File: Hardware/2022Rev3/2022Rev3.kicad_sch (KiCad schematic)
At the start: 101 parts, among them J1 Conn_01x04, J2 Conn_01x06, J3 RJ45_LED_Shielded, J4 Conn_01x09, J5 Conn_01x09, J6 Conn_01x03, Q1 Q_NMOS_DGS, Q2 Q_NMOS_DGS, SW1 SW_SPDT, U1 ACS758xCB-200B-PFF, U2 LT1910, U3 TRS12433, U4 TRS12450, U5 Teensy4.1_DEV-16771, U6 Opamp_Dual, U7 Opamp_Dual, U8 Opamp_Dual, U9 Opamp_Dual

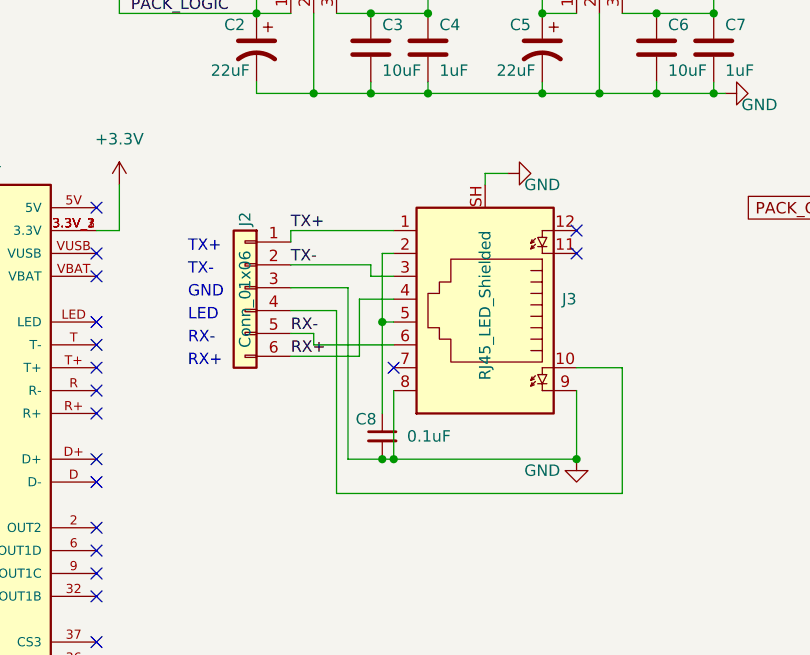
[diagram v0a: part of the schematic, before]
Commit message: layout changes
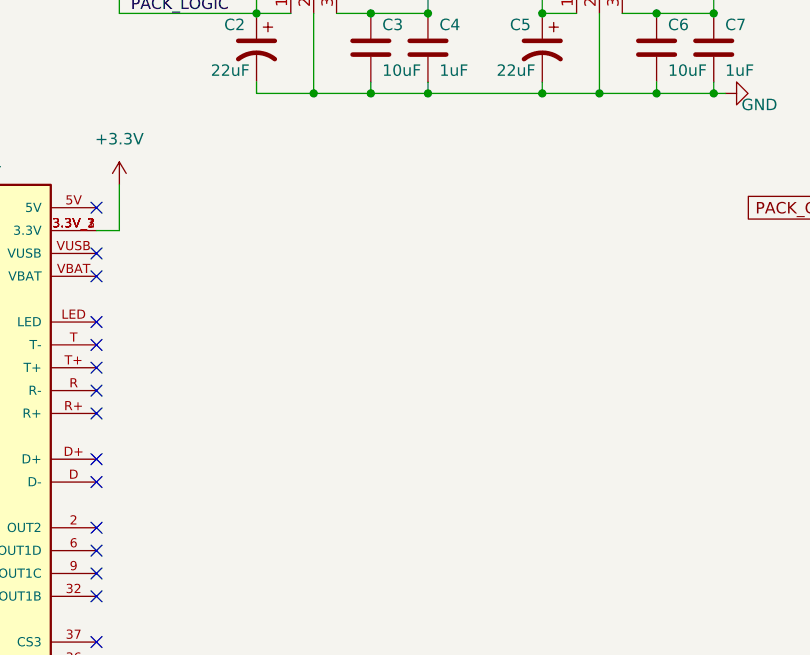
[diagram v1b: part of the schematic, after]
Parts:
- removed C8: 0.1uF, Capacitor_SMD:C_0603_1608Metric_Pad1.08x0.95mm_HandSolder, symbol Device:C_Small
- removed J2: Conn_01x06, Connector_PinHeader_2.00mm:PinHeader_2x03_P2.00mm_Vertical, symbol Connector_Generic:Conn_01x06
- removed J3: RJ45_LED_Shielded, MRDT_Connectors:RJ45_Teensy, symbol Connector:RJ45_LED_Shielded
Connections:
- no-connect marks 47 -> 44
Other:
- note removed: "GND"
- note removed: "LED"
- note removed: "RX+"
- note removed: "RX-"
- note removed: "TX+"
- note removed: "TX-"
